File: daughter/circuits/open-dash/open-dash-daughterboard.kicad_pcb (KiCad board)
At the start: 4 copper layers, 125 x 100.1 mm, 225 parts, among them J1 Conn_01x01_Female, J10 Barrel_Jack_OD5.5_ID2.5, J11 Barrel_Jack_OD5.5_ID2.5, J12 AudioJack_3.5TRS, J13 AudioJack_3.5TRS, J14 Conn_02x03_Odd_Even, J15 USB_MINI_B, J16 Conn_02x02_Counter_Clockwise, J2 Conn_01x01_Female, J3 Conn_01x01_Female, J4 Conn_01x01_Female, J42 Terminal_01x04, J43 Conn_02x02_Counter_Clockwise, J44 Terminal_01x04, J45 Terminal_01x04, J46 Conn_02x02_Counter_Clockwise, J5 Conn_02x06_Odd_Even, J6 Conn_IDE_40, J7 Conn_IDE_40, J8 Conn_IDE_40, J9 Barrel_Jack_OD5.5_ID2.5, Q1 Crystal_12Mhz, Q10 Q_NPN_BEC, Q11 Q_AO3401A, Q12 Q_NPN_BEC, Q13 Q_NPN_BEC, Q14 Q_AO3400A, Q15 Q_NPN_BEC, Q16 Q_NPN_BEC, Q17 Q_AO3401A, Q18 Q_NPN_BEC, Q19 Q_NPN_BEC, Q2 Q_SS8050, Q20 Q_AO3400A, Q21 Q_NPN_BEC, Q22 Q_NPN_BEC, Q23 Q_AO3401A, Q24 Q_AO3400A, Q25 Q_AO3401A, Q26 Q_AO3400A, Q27 Q_AO3401A, Q28 Q_AO3400A, Q29 Q_AO3401A, Q3 Q_NPN_BEC, Q30 Q_AO3400A, Q31 Q_AO3401A, Q32 Q_AO3400A, Q33 Q_AO3401A, Q34 Q_AO3400A, Q35 Q_AO3401A, Q36 Q_AO3400A, Q37 Q_AO3401A, Q38 Q_AO3400A, Q39 Q_SS8550, Q4 Q_NPN_BEC, Q40 Q_AO3401A, Q5 Q_NPN_BEC, Q6 Q_NPN_BEC, Q7 Q_NPN_BEC, Q8 Q_NPN_BEC, Q9 Q_NPN_BEC, T1 Audio_Transformer, T2 Audio_Transformer, T3 Audio_Transformer, T4 Audio_Transformer, U1 Opto_TLP521, U10 Temp_Hum_HDC1080DMBR, U11 REG_AMS1117-3.3, U12 CH340T(SSOP20W), U13 MCP23017_SS, U14 ADC_ADS1015, U15 ADC_ADS1015, U16 ADC_ADS1015, U2 ACS711, U3 CAN_MCP2551-I-SN, U4 MIC29302WU, U5 MIC29302WU, U6 MIC29302WU, U7 TDA7851F, U8 Opto_TLP521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

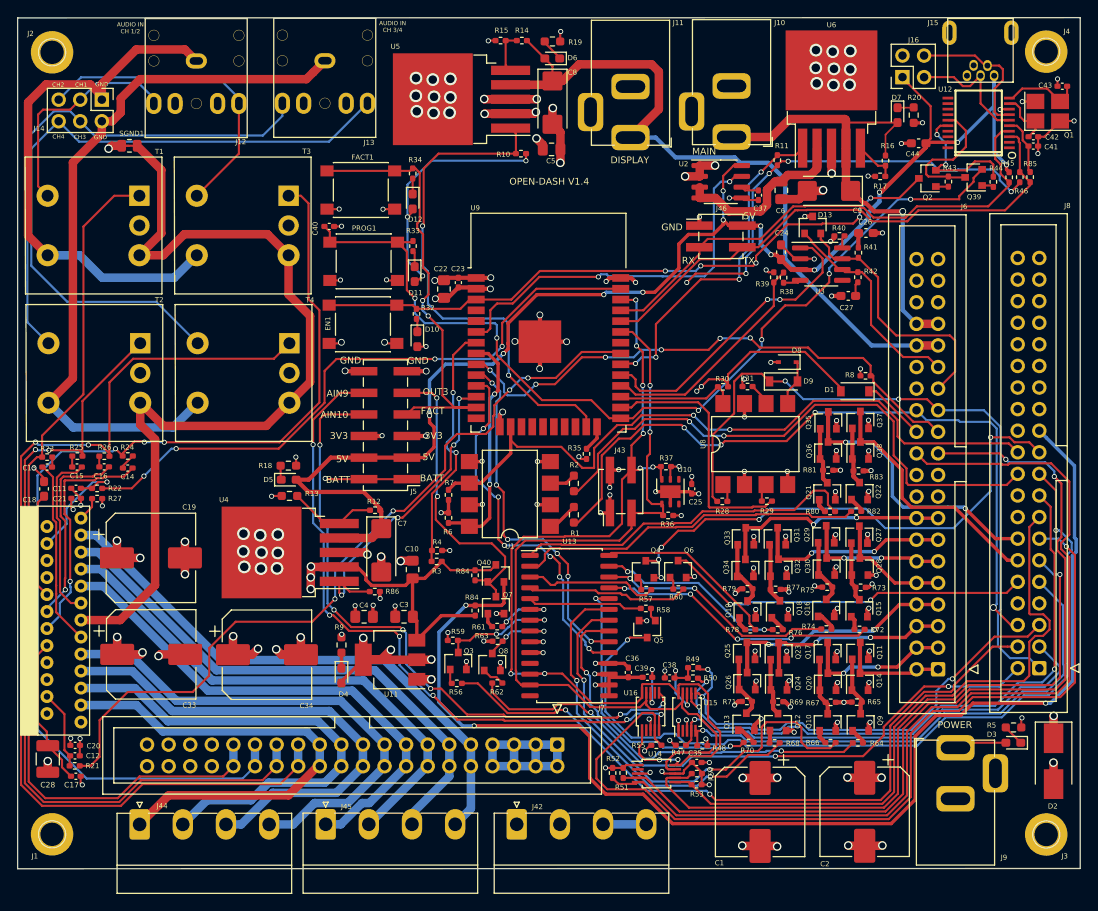
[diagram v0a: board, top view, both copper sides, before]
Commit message: Updated schematic
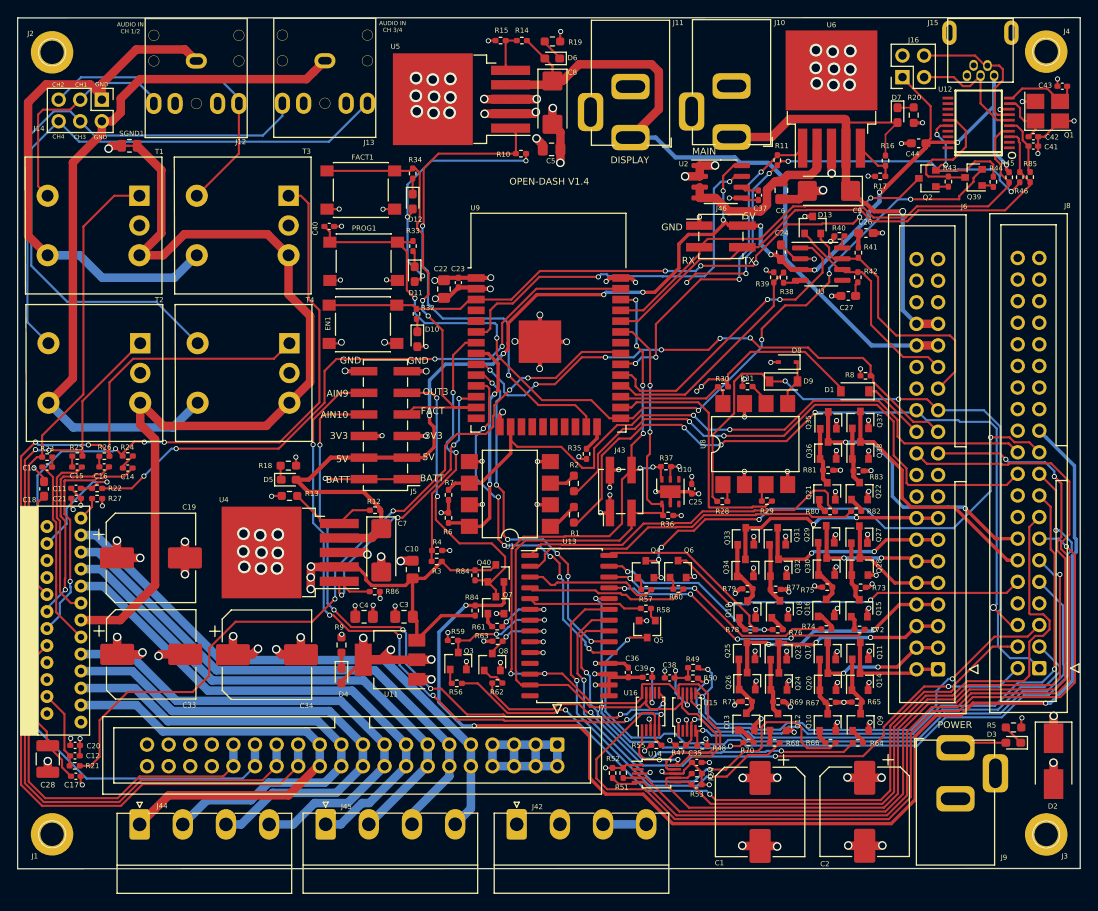
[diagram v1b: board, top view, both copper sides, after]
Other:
- net class Default removed
- net class HIGH CURRENT removed
- net class LOW CURRENT removed
- net class MED CURRENT removed
